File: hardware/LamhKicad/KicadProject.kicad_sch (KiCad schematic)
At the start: 53 parts, among them J1 JTAG-10 PIN, J2 436500303, J3 436500303, J4 436500303, J5 ESQ-110-X-X-D, J6 436500303, U1 TJA1051T-3, U2 PCA9685PW_112, U3 TLV70433DBVT, U4 STM32F072C8Tx

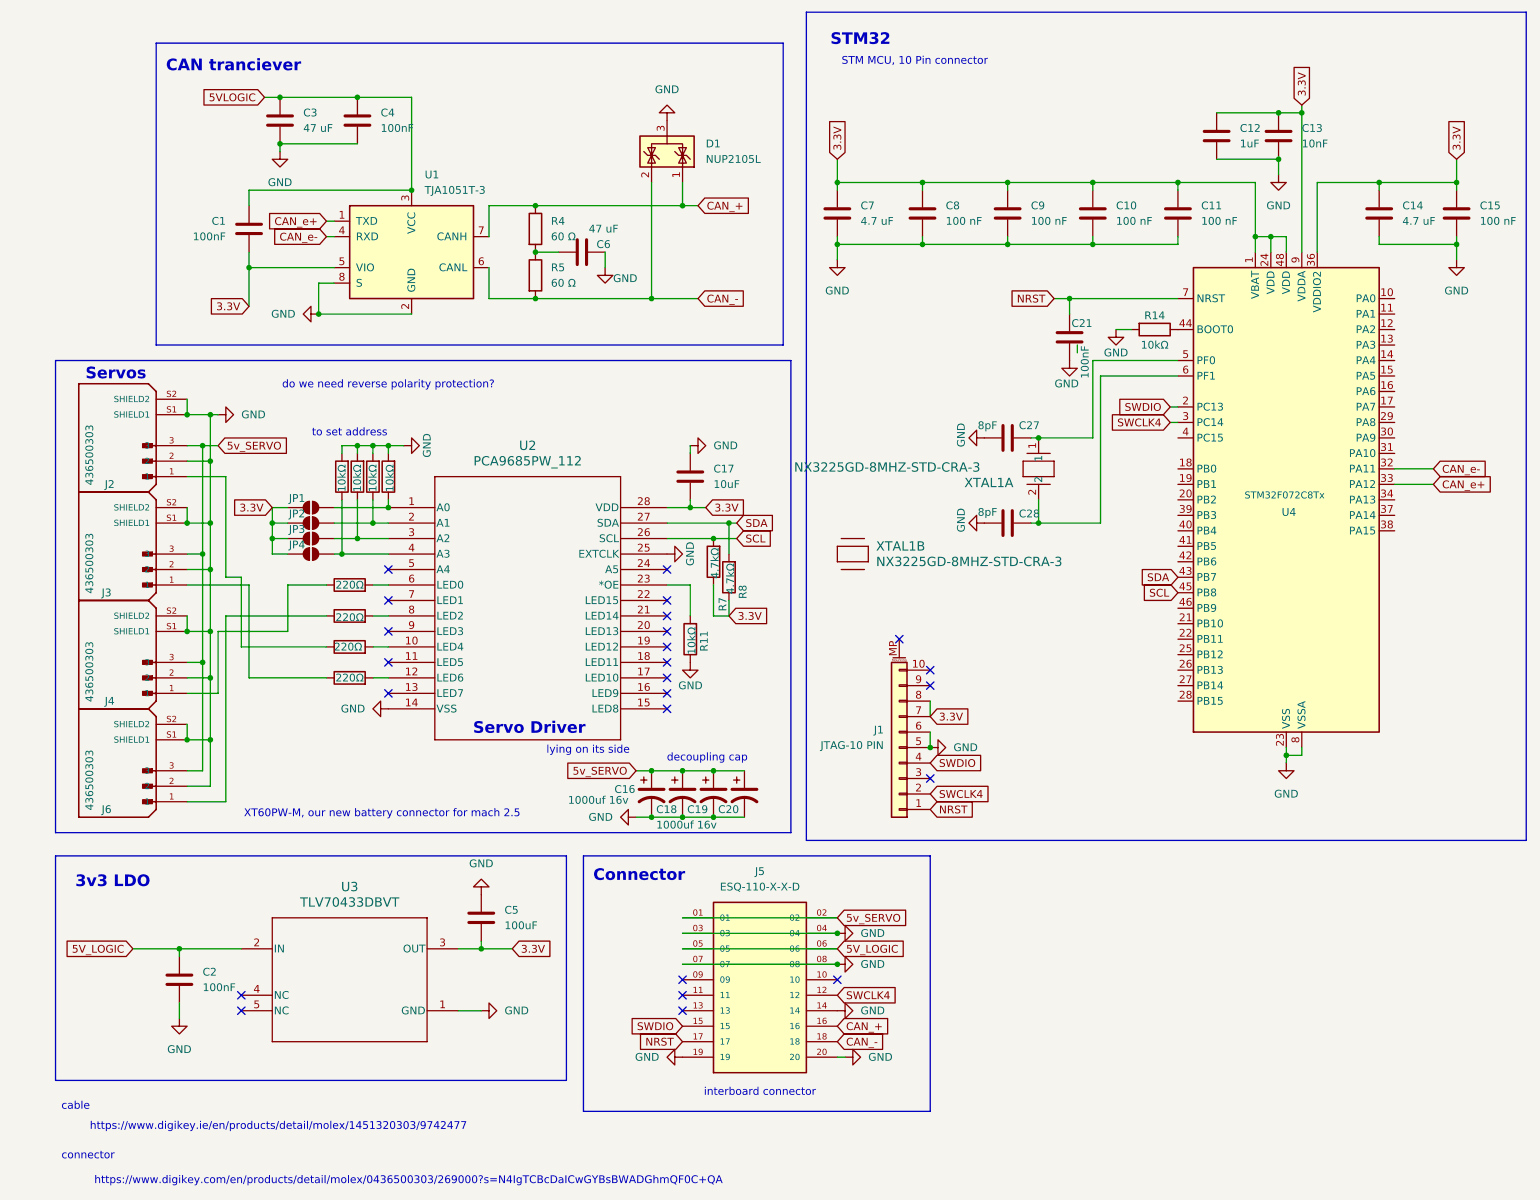
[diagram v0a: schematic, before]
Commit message: mockup done, must finish routing
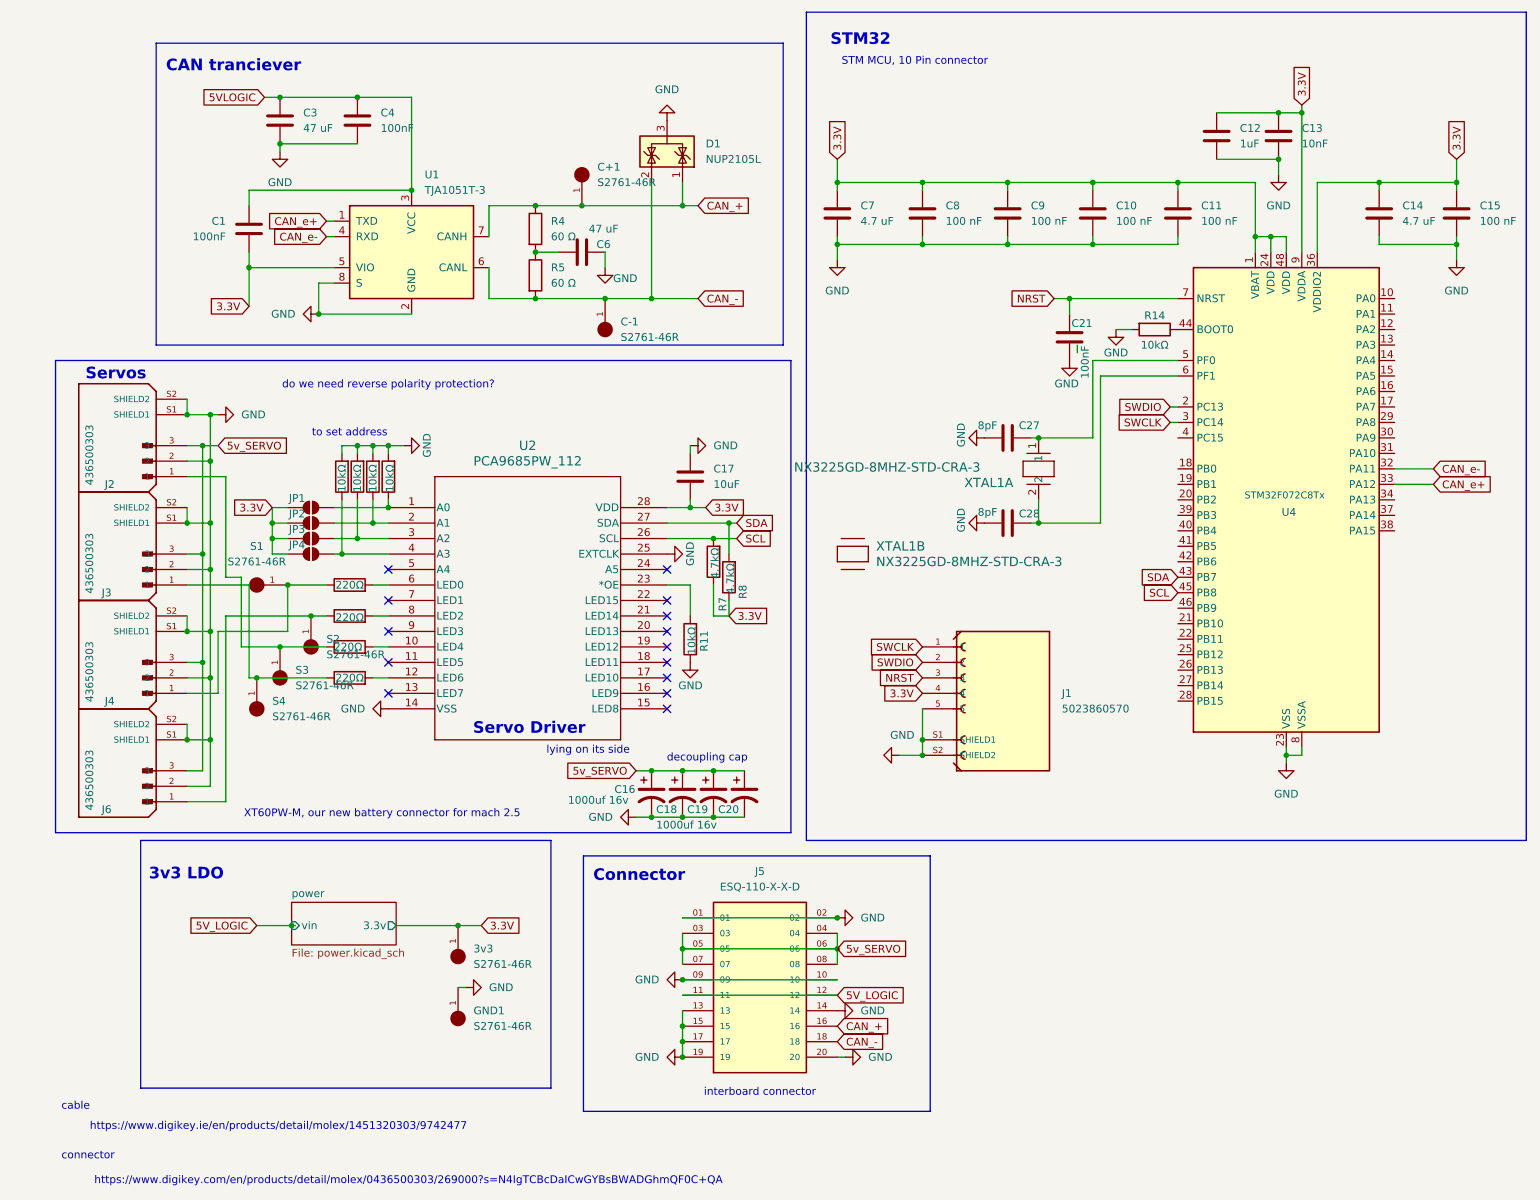
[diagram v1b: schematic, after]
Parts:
- removed C2: 100nF, Capacitor_SMD:C_0402_1005Metric, symbol Device:C
- removed C5: 100uF, Capacitor_SMD:C_0402_1005Metric, symbol Device:C
- removed J1: JTAG-10 PIN, Connector_IDC:IDC-Header_2x05_P2.54mm_Vertical, symbol Connector_Generic_MountingPin:Conn_01x10_MountingPin
- removed U3: TLV70433DBVT, DBV0005A_N, symbol TLV70433DBVT:TLV70433DBVT
- added 3v3, C+1, C-1, GND1, S1, S2, S3, S4: S2761-46R, HARWIN_S2761-46R, symbol S2761-46R:S2761-46R
- added J1: 5023860570, MOLEX_5023860570, symbol 5023860570:5023860570
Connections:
- net 3.3V: now also 3v3.1, J1.4
- net 5V_LOGIC: now also J5.11, J5.12; no longer J5.05, J5.06
- net 5v_SERVO: now also J5.03, J5.04, J5.05, J5.06, J5.07, J5.08; no longer J5.01, J5.02
- net CAN_+: now also C+1.1
- net CAN_-: now also C-1.1
- net GND: now also J5.01, J5.02, J5.09, J5.10, J5.13, J5.15, J5.17, GND1.1, J1.5, J1.S1 (SHIELD1), J1.S2 (SHIELD2); no longer J5.03, J5.04, J5.07, J5.08
- net NRST: now also J1.3; no longer J5.17
- net SWDIO: now also J1.2; no longer J5.15
- net at J2.1, R3.1: now also S3.1
- net at J3.1, R6.1: now also S4.1
- net at J6.1, R2.1: now also S2.1
- net at J4.1, R1.1: now also S1.1
- net SWCLK4 renamed SWCLK
- net SWCLK: now also J1.1; no longer J5.12
- no-connect marks 24 -> 14
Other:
- added sheet power (power.kicad_sch)

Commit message: clean asf
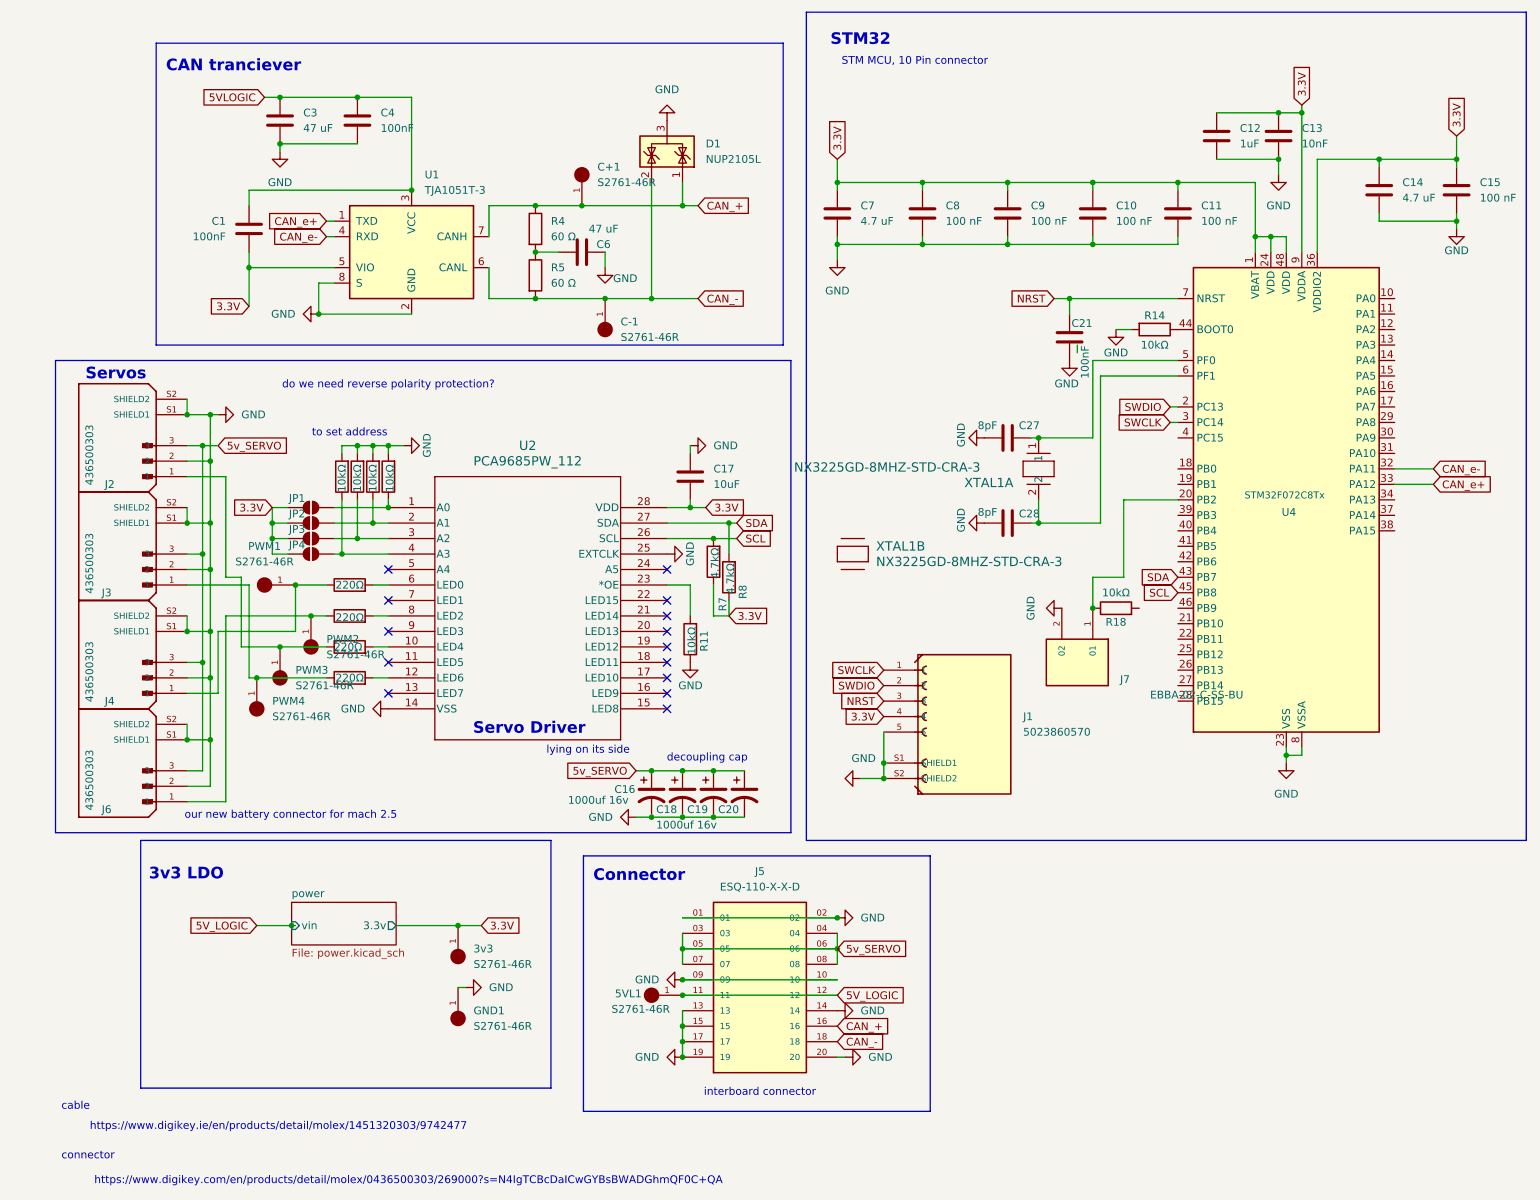
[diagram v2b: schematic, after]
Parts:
- added 5VL1: S2761-46R, HARWIN_S2761-46R, symbol S2761-46R:S2761-46R
- added J7: EBBA-02-C-SS-BU, EBBA-02-C-SS-BU, symbol EBBA-02-C-SS-BU:EBBA-02-C-SS-BU
- added R18: 10kΩ, Resistor_SMD:R_0402_1005Metric, symbol Device:R
- renumbered S1 to PWM1, S2 to PWM2, S3 to PWM3, S4 to PWM4
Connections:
- net 5V_LOGIC: now also 5VL1.1
- net GND: now also J7.2 (02)
- net at U4.20 (PB2): now also J7.1 (01), R18.1
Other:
- note added: "our new battery connector for mach 2.5"
- note removed: "XT60PW-M, our new battery connector for mach 2.5"
- moved on the sheet: C14, C15, J1, PWM1
